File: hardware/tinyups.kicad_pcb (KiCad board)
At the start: 4 copper layers, 144.6 x 137.5 mm, 122 parts, among them J1 XT60, J2 XT30, J3 USB, J4 SWD, J5 FAN, Q1 N-FET 40V, Q10 N-FET 40V, Q11 N-FET 40V, Q12 N-FET 40V, Q2 N-FET 40V, Q3 N-FET 30V, Q4 N-FET 30V, Q5 N-FET 30V, Q6 N-FET 30V, Q7 N-FET 40V, Q8 N-FET 40V, Q9 N-FET 40V, U1 LM5069, U2 LM74700-Q1, U3 BQ25720, U4 LM5176, U5 BQ76942, U6 RP2040, U7 W25Q128, U8 3V3, Y1 12MHz

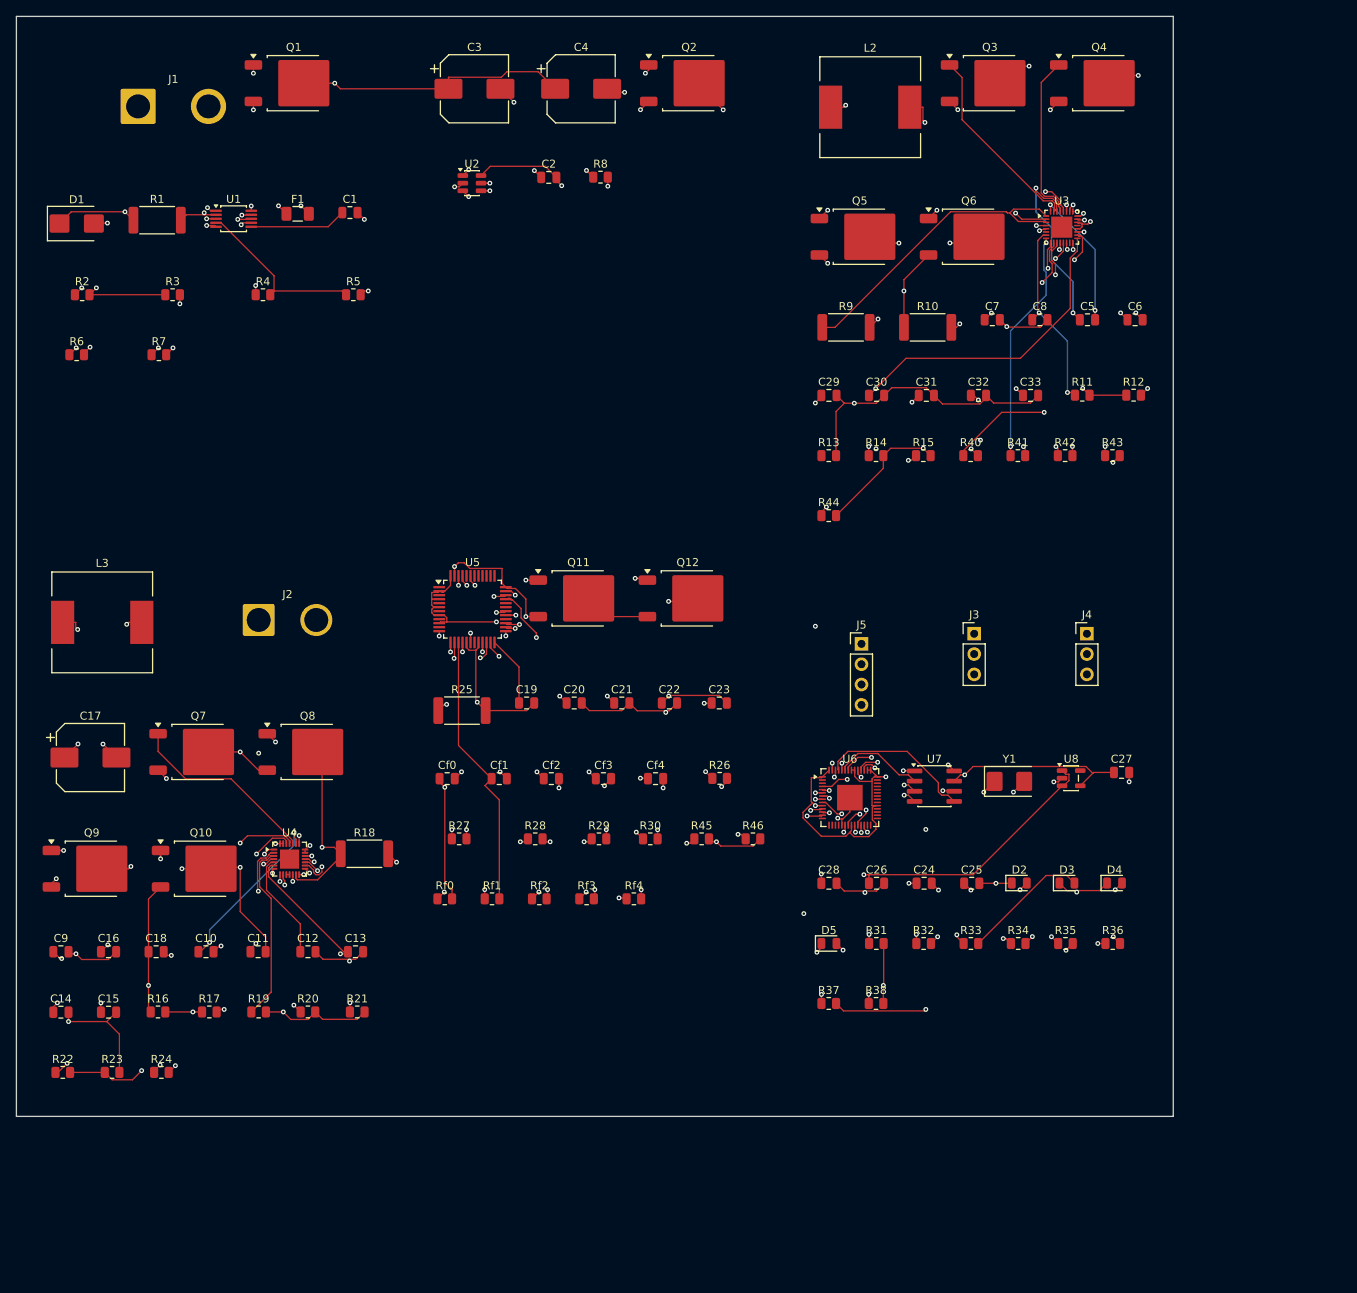
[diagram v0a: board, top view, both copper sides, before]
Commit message: work on routing. llm hit wall
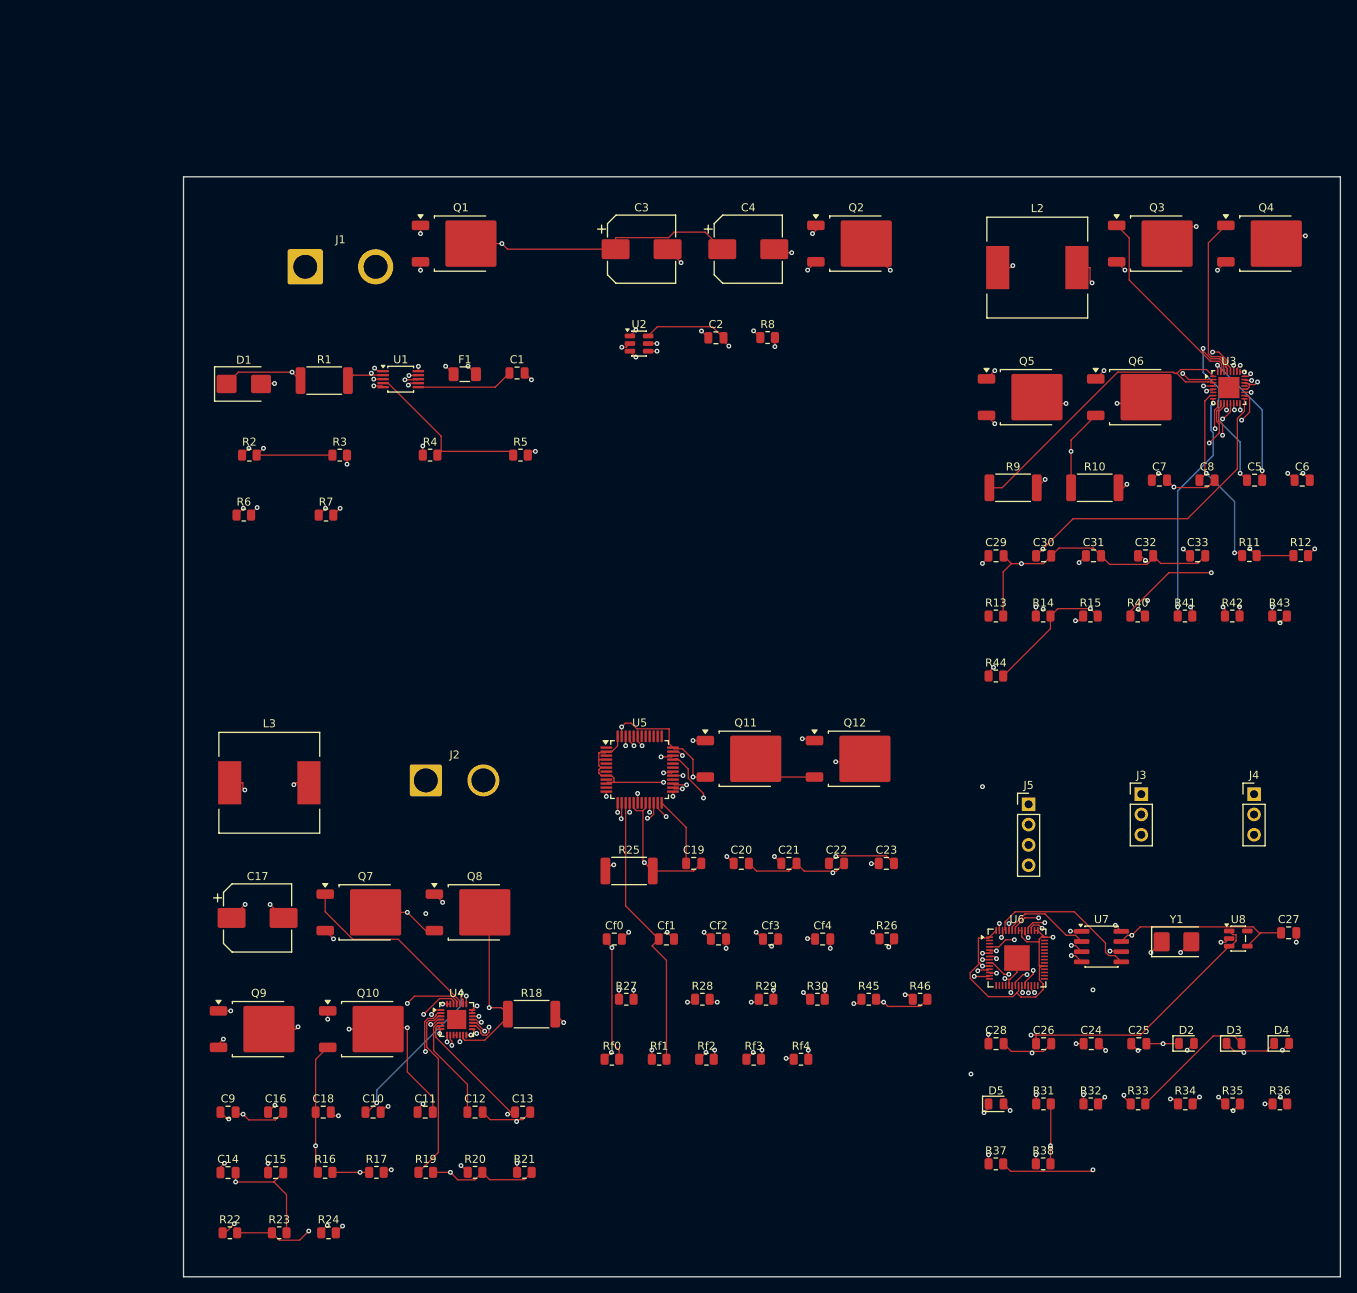
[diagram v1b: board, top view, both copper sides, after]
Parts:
- moved J4 29.0 mm to (153.9, 97.2)
- moved U7 29.0 mm to (134.8, 116.3)
- moved U8 29.0 mm to (151.9, 115.3)
- moved C5 29.0 mm to (153.9, 58.0)
- moved Q6 29.0 mm to (139.1, 47.6)
- moved Cf0 29.0 mm to (73.9, 115.3)
- moved Cf1 29.0 mm to (80.4, 115.3)
- moved Cf2 29.0 mm to (86.9, 115.3)
- moved Cf4 29.0 mm to (99.9, 115.3)
- moved D3 29.0 mm to (151.4, 128.4)
- moved J2 29.0 mm to (50.3, 95.5)
- moved J3 29.0 mm to (139.8, 97.2)
- moved R18 29.0 mm to (63.6, 124.7)
- moved R33 29.0 mm to (139.4, 135.9)
- moved R35 29.0 mm to (151.2, 135.9)
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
